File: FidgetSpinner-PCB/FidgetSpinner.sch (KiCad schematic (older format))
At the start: 38 parts, among them J1 EdgeConnector, Q1 Q_Photo_NPN, SW1 SW_POWER, SW2 button, U1 STM32L010K8T6

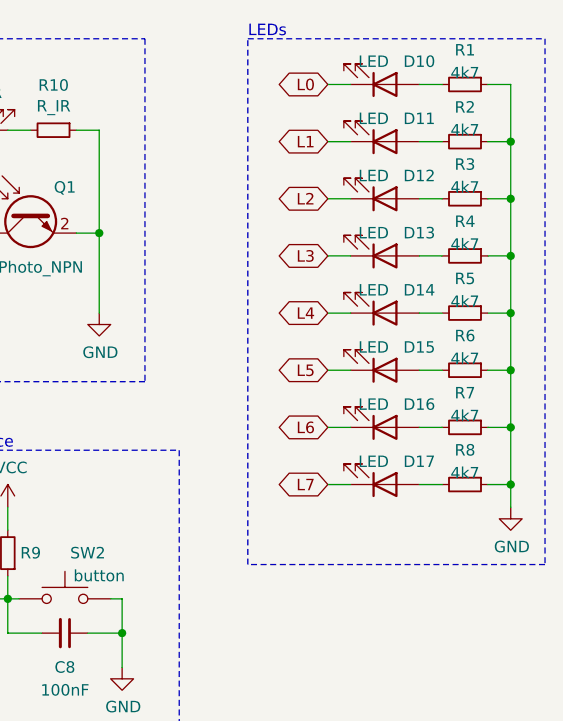
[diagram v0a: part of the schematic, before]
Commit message: backup of CLion project
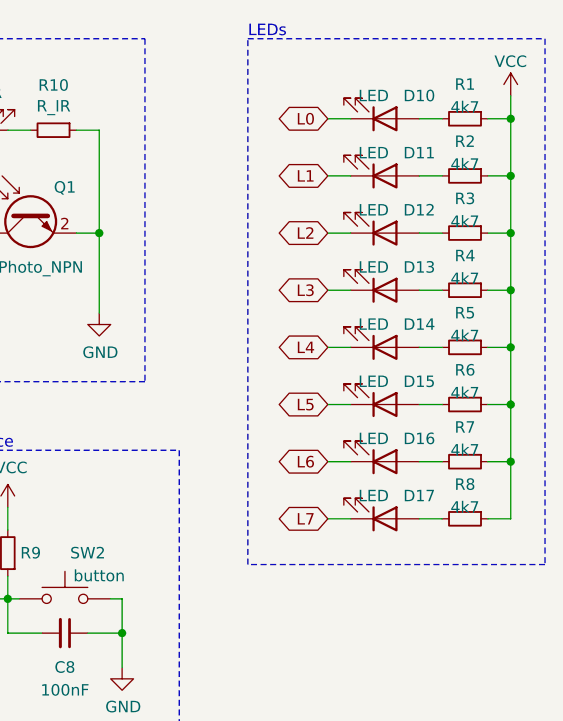
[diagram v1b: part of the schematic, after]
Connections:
- net GND: no longer R1.1, R2.1, R3.1, R4.1, R5.1, R6.1, R7.1, R8.1
- net VCC: now also R1.1, R2.1, R3.1, R4.1, R5.1, R6.1, R7.1, R8.1
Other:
- moved on the sheet: D10, D11, D12, D13, D14, D15, D16, D17, R1, R2, R3, R4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
